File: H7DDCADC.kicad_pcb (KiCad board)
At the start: 4 copper layers, 134 x 71 mm, 167 parts, among them J1 U.FL-DNP, J2 SMA, J3 SMA, J4 HDR2, J5 HDR2x4, J6 HDR2, J7 HDR3, J8 HDR2, J9 HDR3, U1 74AUC1G74DCT, U10 74AUC2G79DCT, U11 74AUC1G08DBV, U12 74AUC1G74DCT, U13 TXB0104D, U14 Si5351A-B-GT, U15 74AUP1T97GW, U16 NUCLEO144-H743ZI, U17 74AUP1T97GW, U18 74AUP1T97GW, U19 74AUP1T97GW, U2 74AUC1G74DCT, U20 74AUP1T97GW, U21 74AUP1T97GW, U23 AP2127K-1.8, U24 AP2127K-1.8, U25 AP2127K-1.8, U3 ADC3660IRSBT, U4 74AUC2G34DBV, U5 74AUC2G34DBV, U6 74AUC2G34DBV, U7 74AUP1T97GW, U8 74AUC1G74DCT, U9 74AUC2G79DCT, X1 SG-7050CAN, Y1 25/27MHz-3225-DNP

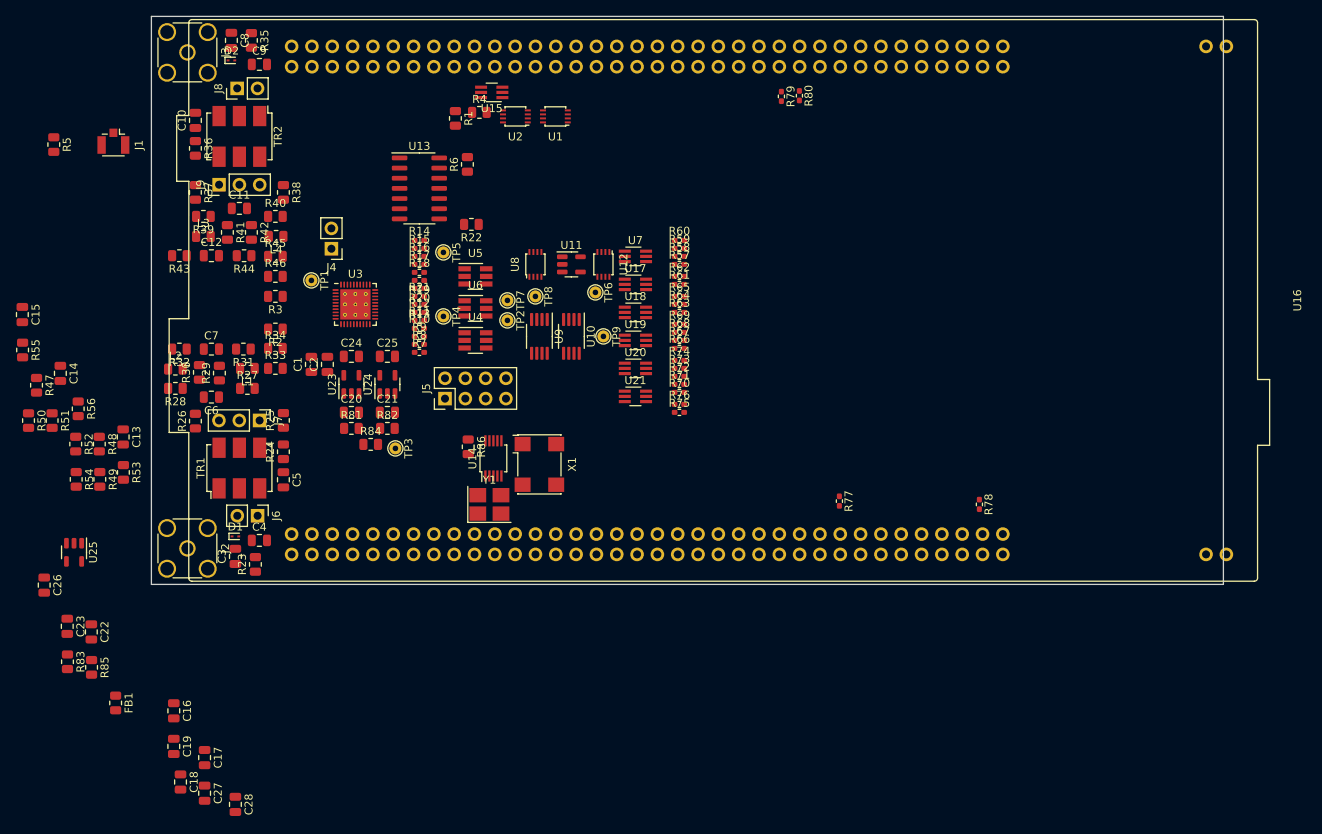
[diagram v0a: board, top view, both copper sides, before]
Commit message: routing in progress 1
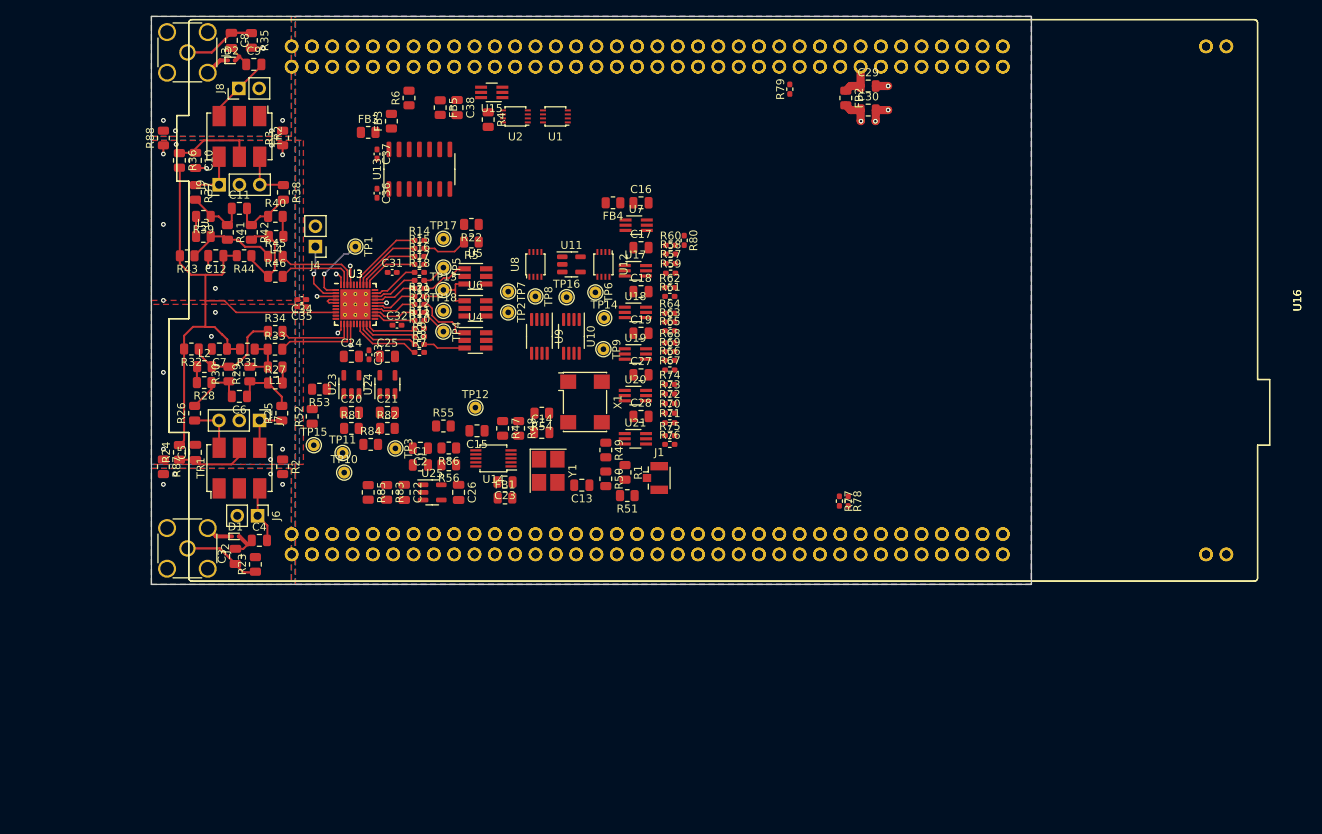
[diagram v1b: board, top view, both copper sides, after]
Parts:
- removed J5: HDR2x4, Connector_PinHeader_2.54mm:PinHeader_2x04_P2.54mm_Vertical
- added C29: 1uF, Capacitor_SMD:C_0805_2012Metric, F.Cu at (176.6, 62.7)
- added C30: 1uF, Capacitor_SMD:C_0805_2012Metric, F.Cu at (176.6, 65.7)
- added C31: 100n, Capacitor_SMD:C_0402_1005Metric_Pad0.74x0.62mm_HandSolder, F.Cu at (117.1, 86.0)
- added C32: 100n, Capacitor_SMD:C_0402_1005Metric_Pad0.74x0.62mm_HandSolder, F.Cu at (117.7, 92.6)
- added C33: 100n, Capacitor_SMD:C_0402_1005Metric_Pad0.74x0.62mm_HandSolder, F.Cu at (114.2, 96.3)
- added C34: 100n, Capacitor_SMD:C_0402_1005Metric_Pad0.74x0.62mm_HandSolder, F.Cu at (105.8, 89.4)
- added C35: 100n, Capacitor_SMD:C_0402_1005Metric_Pad0.74x0.62mm_HandSolder, F.Cu at (105.8, 90.3)
- added C36: 100n, Capacitor_SMD:C_0402_1005Metric_Pad0.74x0.62mm_HandSolder, F.Cu at (115.2, 76.1)
- added C37: 100n, Capacitor_SMD:C_0402_1005Metric_Pad0.74x0.62mm_HandSolder, F.Cu at (115.2, 71.2)
- added C38: 100nF, Capacitor_SMD:C_0805_2012Metric, F.Cu at (125.2, 65.4)
- added FB2: Ferrite_0805, Resistor_SMD:R_0805_2012Metric, F.Cu at (173.8, 64.2)
- added FB3: Ferrite_0805, Resistor_SMD:R_0805_2012Metric, F.Cu at (114.1, 68.5)
- added FB3: Ferrite_0805, Resistor_SMD:R_0805_2012Metric, F.Cu at (117.0, 67.1)
- added FB4: Ferrite_0805, Resistor_SMD:R_0805_2012Metric, F.Cu at (144.7, 77.3)
- added FB5: Ferrite_0805, Resistor_SMD:R_0805_2012Metric, F.Cu at (123.1, 65.4)
- added R87: 0R, Resistor_SMD:R_0805_2012Metric, F.Cu at (88.5, 110.3)
- added R88: 0R, Resistor_SMD:R_0805_2012Metric, F.Cu at (88.5, 69.2)
- added TP10: CLKP_ADC, TestPoint:TestPoint_THTPad_D1.5mm_Drill0.7mm, F.Cu at (111.1, 111.0)
- added TP11: CLKN_ADC, TestPoint:TestPoint_THTPad_D1.5mm_Drill0.7mm, F.Cu at (110.9, 108.6)
- added TP12: DCLK_IN_D3, TestPoint:TestPoint_THTPad_D1.5mm_Drill0.7mm, F.Cu at (127.5, 102.9)
- added TP13: DCLK_ADC, TestPoint:TestPoint_THTPad_D1.5mm_Drill0.7mm, F.Cu at (123.5, 88.2)
- added TP14: GND, TestPoint:TestPoint_THTPad_D1.5mm_Drill0.7mm, F.Cu at (143.6, 91.7)
- added TP15: GND, TestPoint:TestPoint_THTPad_D1.5mm_Drill0.7mm, F.Cu at (107.3, 107.6)
- added TP16: GND, TestPoint:TestPoint_THTPad_D1.5mm_Drill0.7mm, F.Cu at (138.9, 89.1)
- added TP17: GND, TestPoint:TestPoint_THTPad_D1.5mm_Drill0.7mm, F.Cu at (123.5, 81.8)
- added TP18: GND, TestPoint:TestPoint_THTPad_D1.5mm_Drill0.7mm, F.Cu at (123.5, 90.8)
- added U16: NUCLEO144-H743ZI_DM1CR, Module:ST_Morpho_Connector_144_STLink, F.Cu at (193.4, 57.8)
- added U3: ADC3660IRSBT, Package_DFN_QFN:QFN-40-1EP_5x5mm_P0.4mm_EP3.6x3.6mm, F.Cu at (112.5, 90.0)
- moved C16 86.3 mm to (148.2, 77.3), turned to 0 degrees
- moved C18 84.1 mm to (148.2, 88.4), turned to 0 degrees
- moved C17 83.9 mm to (148.2, 82.9), turned to 0 degrees
- moved J1 79.8 mm to (150.0, 111.7), turned to 0 degrees
- moved C19 78.0 mm to (148.2, 93.6), turned to 0 degrees
- moved C27 75.6 mm to (148.2, 98.8), turned to 0 degrees
- moved R50 72.5 mm to (143.8, 111.8)
- moved R51 72.5 mm to (146.5, 113.9), turned to 180 degrees
- moved C28 70.2 mm to (148.2, 104.0), turned to 0 degrees
- moved R49 63.4 mm to (143.8, 108.2)
- moved C14 60.6 mm to (135.8, 106.0), turned to 0 degrees
- moved R54 58.8 mm to (135.8, 103.6), turned to 180 degrees
- moved C15 58.7 mm to (127.7, 105.8), turned to 180 degrees
- moved R47 58.5 mm to (130.9, 105.5)
- moved C13 57.6 mm to (140.8, 112.6), turned to 180 degrees
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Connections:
- C16 pad 1: +3V3 -> V1T97
- C17 pad 1: +3V3 -> V1T97
- C18 pad 1: +3V3 -> V1T97
- C19 pad 1: +3V3 -> V1T97
- C20 pad 1: +3V3 -> +3.3VF
- C21 pad 1: +3V3 -> +3.3VF
- C22 pad 1: +3V3 -> +3.3VF
- C27 pad 1: +3V3 -> V1T97
- C28 pad 1: +3V3 -> V1T97
- FB1 pad 1: +3V3 -> +3.3VF
- R80 pad 2: /MCU/I2C1_SDA_A -> /MCU/SPI2_NSS_D
- R81 pad 1: +3V3 -> +3.3VF
- R82 pad 1: +3V3 -> +3.3VF
- R83 pad 1: +3V3 -> +3.3VF
- U13 pad 14: +3V3 -> Net-(C37-Pad1)
- U15 pad 5: +3V3 -> VEXTCLK
- U17 pad 5: +3V3 -> V1T97
- U18 pad 5: +3V3 -> V1T97
- U19 pad 5: +3V3 -> V1T97
- U20 pad 5: +3V3 -> V1T97
- U21 pad 5: +3V3 -> V1T97
- U23 pad 1: +3V3 -> +3.3VF
- U24 pad 1: +3V3 -> +3.3VF
- U25 pad 1: +3V3 -> +3.3VF
- U7 pad 5: +3V3 -> V1T97
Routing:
- net VCM: track 0.00 -> 68.6 mm
- net GND: track 0.00 -> 21.3 mm, vias 0 -> 24
- net Net-(L2-Pad2): track 0.00 -> 13.0 mm
- net Net-(L3-Pad2): track 0.00 -> 11.6 mm
- net Net-(L4-Pad2): track 0.00 -> 11.5 mm
- net /ADC/AIN_N: track 0.00 -> 10.7 mm
- net Net-(C10-Pad1): track 0.00 -> 10.6 mm
- net /ADC/BIN_N: track 0.00 -> 10.6 mm
- net /ADC/BIN_P: track 0.00 -> 9.89 mm
- net /IN_A_50: track 0.00 -> 9.81 mm
- net /ADC/AIN_P: track 0.00 -> 9.78 mm
- net Net-(R14-Pad1): track 0.00 -> 9.67 mm
- net Net-(C5-Pad1): track 0.00 -> 9.24 mm
- net /IN_B_50: track 0.00 -> 9.03 mm
- net Net-(R7-Pad1): track 0.00 -> 8.78 mm
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- added copper zone on In2.Cu, net +3.3VA
- added copper zone on In2.Cu, net +3.3VF
- added copper zone on B.Cu, net /GNDI_A
- added copper zone on F.Cu, net /GNDI_A
- added copper zone on In1.Cu, net /GNDI_A
- added copper zone on In2.Cu, net /GNDI_A
- added copper zone on B.Cu, net /GNDI_B
- added copper zone on F.Cu, net /GNDI_B
- added copper zone on In1.Cu, net /GNDI_B
- added copper zone on In2.Cu, net /GNDI_B
- added copper zone on B.Cu, net GND
- added copper zone on F.Cu, net GND
- added copper zone on In1.Cu, net GND
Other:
- board size 134 x 71 mm -> 110 x 71 mm
